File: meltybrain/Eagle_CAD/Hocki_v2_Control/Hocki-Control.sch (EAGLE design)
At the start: 148 parts, among them CN1 JST_2PIN, J1 SM03B-SRSS-TB(LF)(SN), J2 SM04B-SRSS-TB(LF)(SN), J4 SM04B-SRSS-TB(LF)(SN), J5 SM03B-SRSS-TB(LF)(SN), J6 SM03B-SRSS-TB(LF)(SN), J7 SM02B-SRSS-TB(LF)(SN), J8 SM02B-SRSS-TB(LF)(SN), U1 AP63200, U10 LMH6612MAX/NOPB, U11 TLV3502AIDCNR, U12 LMH6612MAX/NOPB, U13 TMP235A4DCKR, U14 ADXL375, U15 NL27WZ32USG, U16 ADXL375, U17 ADXL375, U18 NL27WZ32USG, U19 ADXL375, U2 TEENSY_4.1, U20 AD8426ACPZ-WP, U21 LMH6612MAX/NOPB, U22 HMC1052L-TR, U23 LMH6612MAX/NOPB, U24 IRF7509, U3 AP2210K-5.0TRG1, U4 AP2210K-3.3TRG1, U5 TXS0104ED, U6 LDL212PU50R, U7 LMH6612MAX/NOPB, U8 LMH6612MAX/NOPB, U9 TMUX1219DCKR

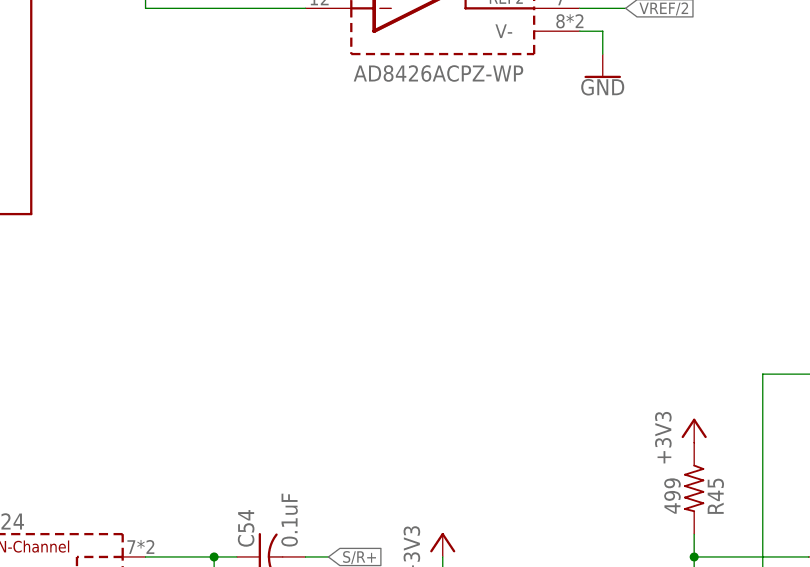
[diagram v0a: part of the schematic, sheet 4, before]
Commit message: add to sch
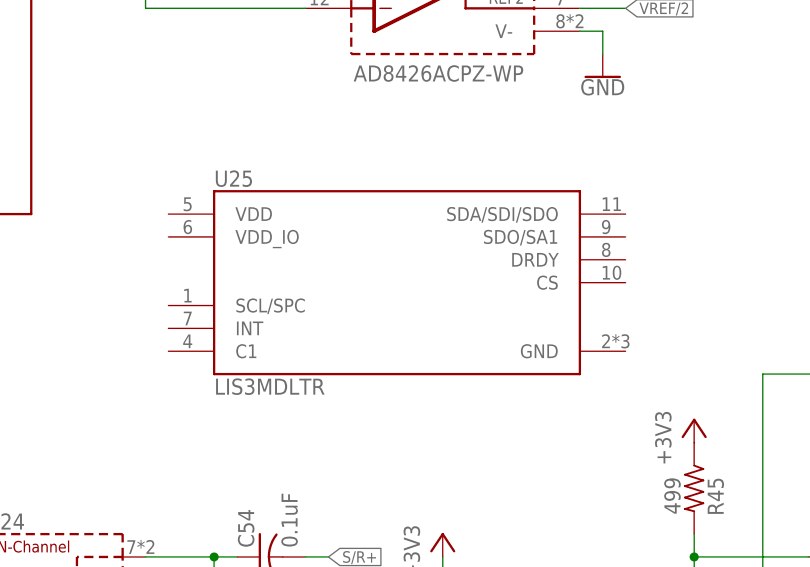
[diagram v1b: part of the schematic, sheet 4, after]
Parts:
- added U25: LIS3MDLTR, Hocki_Library:LIS3MDLTR
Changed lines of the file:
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@@
 <part name="GND83" library="SparkFun-PowerSymbols" deviceset="GND" device=""/>
 <part name="U5" library="Hocki_Library" deviceset="TXS0104ED" device=""/>
+<part name="U25" library="Hocki_Library" deviceset="LIS3MDLTR" device=""/>
 </parts>
 <sheets>
@@
 <attribute name="VALUE" x="184.15" y="173.482" size="1.778" layer="96" rot="R180"/>
 </instance>
+<instance part="U25" gate="A" x="198.12" y="134.62" smashed="yes">
+<attribute name="NAME" x="177.8" y="145.288" size="1.778" layer="95" ratio="6" rot="SR0"/>
+<attribute name="VALUE" x="177.8" y="123.952" size="1.778" layer="96" align="top-left"/>
+</instance>
 </instances>
